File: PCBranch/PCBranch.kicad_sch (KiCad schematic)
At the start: 15 parts, among them J1 CLP-105-02-X-D, J2 DF40HC_3.0_-100DS-0.4V_51_, J3 DF40HC_3.0_-100DS-0.4V_51_, J4 Conn_02x25_Odd_Even, J5 Conn_02x25_Odd_Even, J6 Conn_02x25_Odd_Even, J7 Conn_02x25_Odd_Even

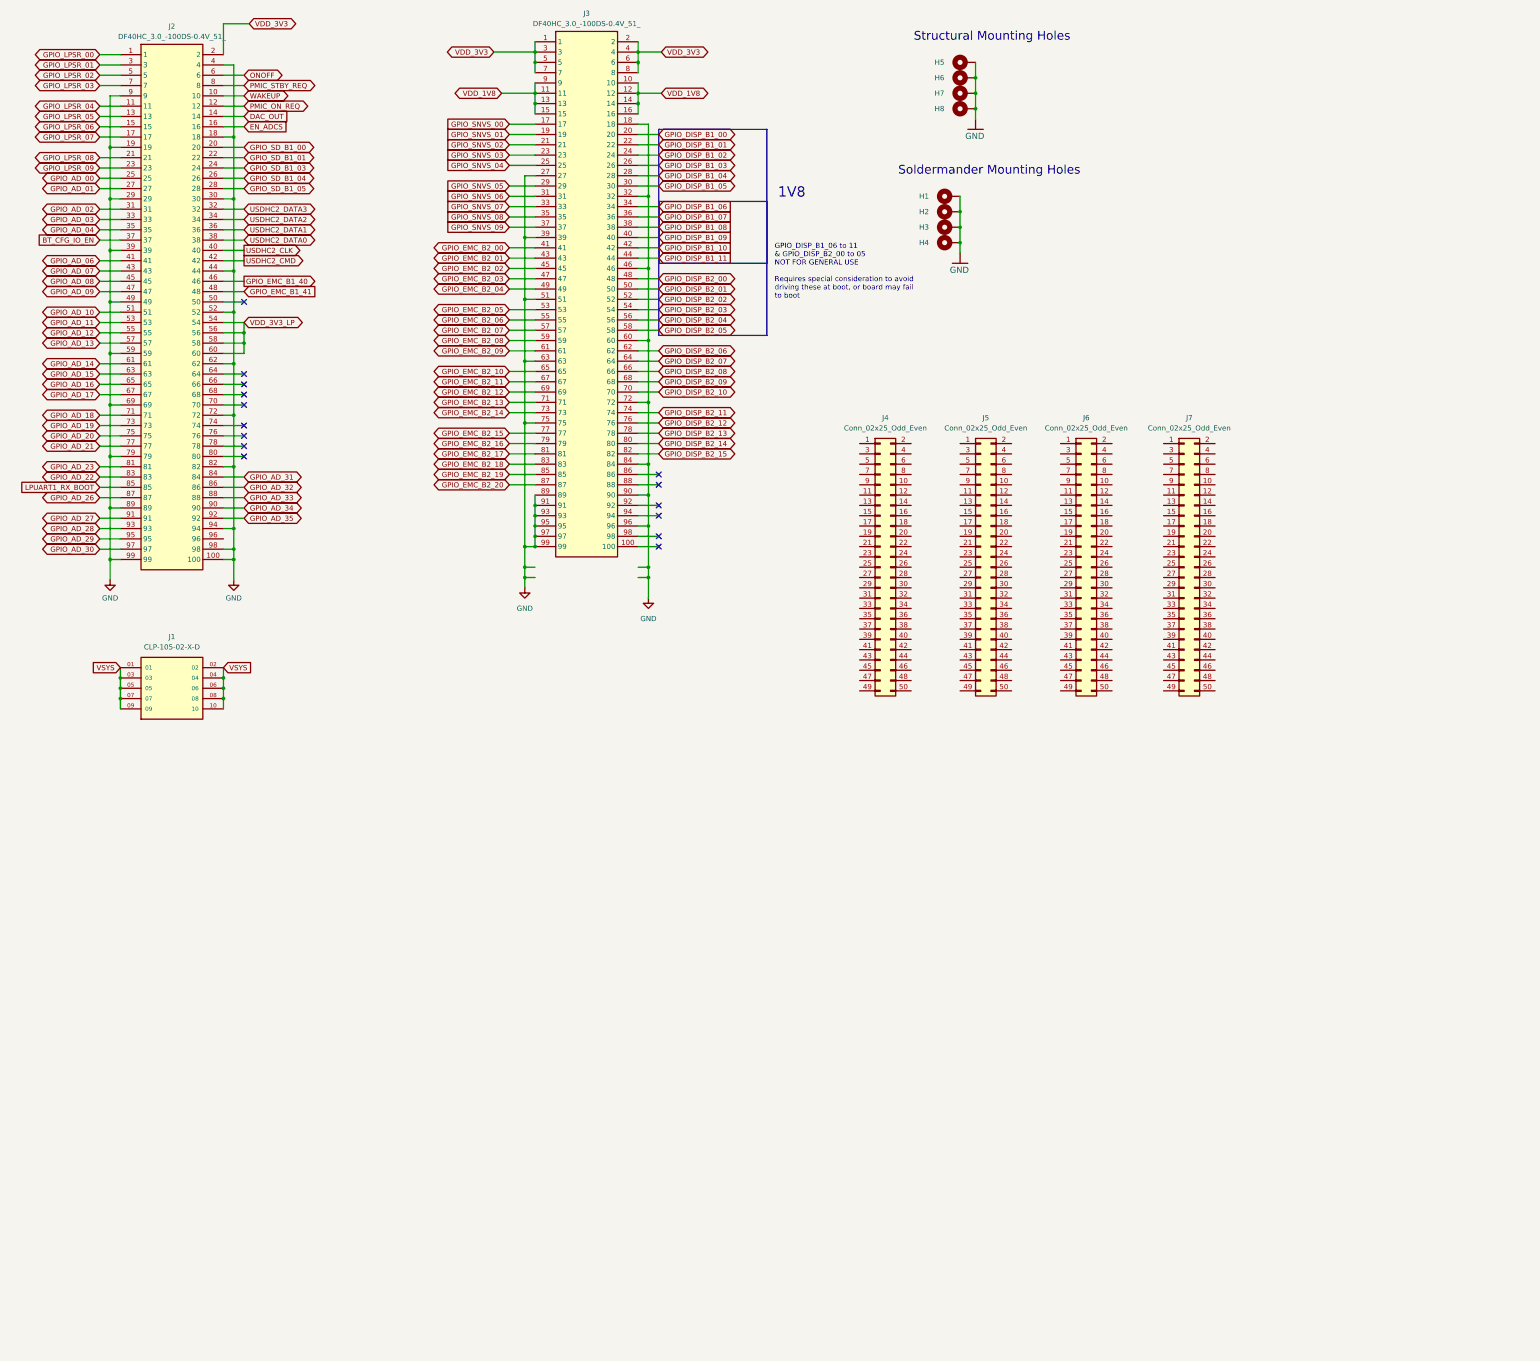
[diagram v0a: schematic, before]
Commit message: PCBranch ready for review
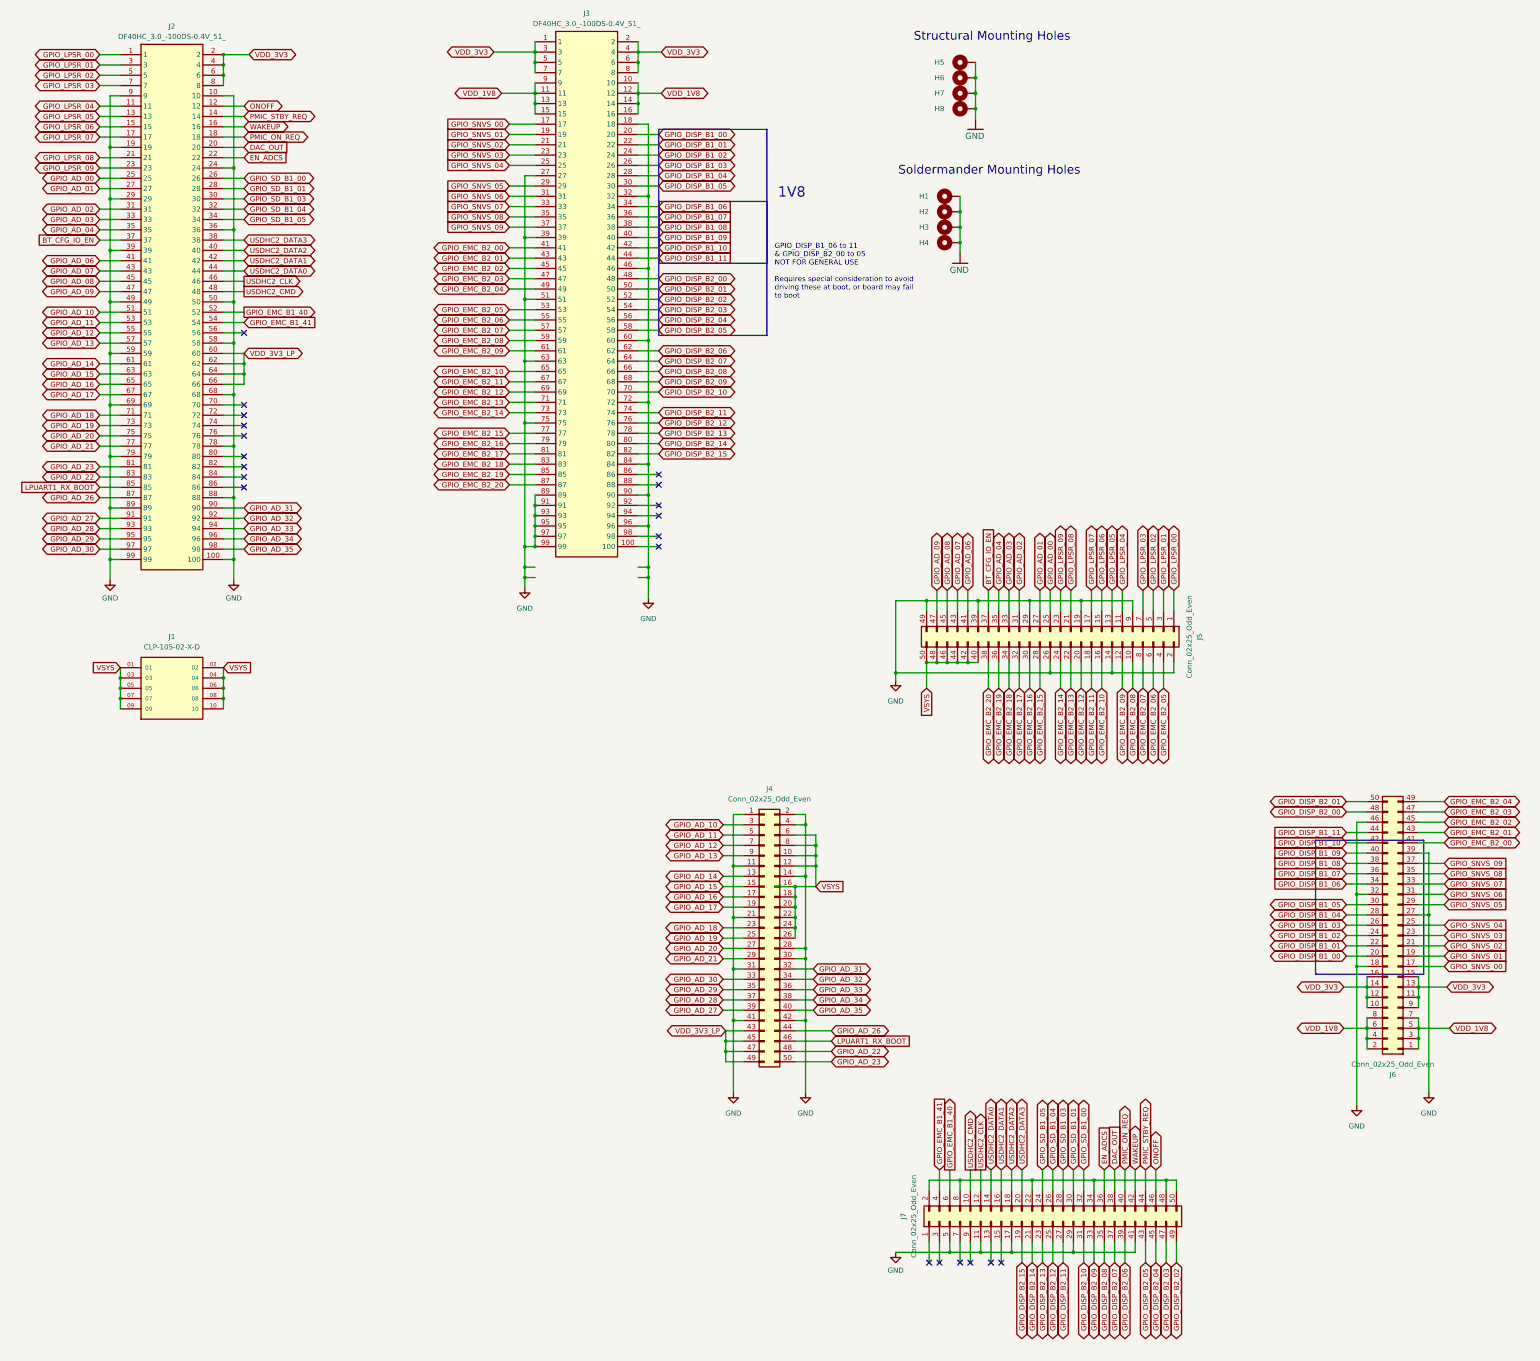
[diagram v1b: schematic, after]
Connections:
- net BT_CFG_IO_EN: now also J5.37 (Pin_37)
- net DAC_OUT: now also J2.20, J7.38 (Pin_38); no longer J2.14
- net EN_ADCS: now also J2.22, J7.36 (Pin_36); no longer J2.16
- net GND: now also J2.10, J2.24, J2.36, J2.50, J2.58, J2.68, J2.78, J2.88, J4.1 (Pin_1), J4.11 (Pin_11), J4.14 (Pin_14), J4.2 (Pin_2), J4.21 (Pin_21), J4.28 (Pin_28), J4.30 (Pin_30), J4.31 (Pin_31), J4.4 (Pin_4), J4.41 (Pin_41), J4.42 (Pin_42), J5.14 (Pin_14), J5.19 (Pin_19), J5.2 (Pin_2), J5.26 (Pin_26), J5.29 (Pin_29), J5.39 (Pin_39), J5.49 (Pin_49), J5.9 (Pin_9), J6.18 (Pin_18), J6.27 (Pin_27), J6.32 (Pin_32), J6.39 (Pin_39), J6.46 (Pin_46), J7.11 (Pin_11), J7.17 (Pin_17), J7.29 (Pin_29), J7.41 (Pin_41), J7.5 (Pin_5); no longer J2.18, J2.30, J2.4, J2.44, J2.52, J2.62, J2.72, J2.82, J2.94, J2.98
- net GPIO_AD_00: now also J5.25 (Pin_25)
- net GPIO_AD_01: now also J5.27 (Pin_27)
- net GPIO_AD_02: now also J5.31 (Pin_31)
- net GPIO_AD_03: now also J5.33 (Pin_33)
- net GPIO_AD_04: now also J5.35 (Pin_35)
- net GPIO_AD_06: now also J5.41 (Pin_41)
- net GPIO_AD_07: now also J5.43 (Pin_43)
- net GPIO_AD_08: now also J5.45 (Pin_45)
- net GPIO_AD_09: now also J5.47 (Pin_47)
- net GPIO_AD_10: now also J4.3 (Pin_3)
- net GPIO_AD_11: now also J4.5 (Pin_5)
- net GPIO_AD_12: now also J4.7 (Pin_7)
- net GPIO_AD_13: now also J4.9 (Pin_9)
- net GPIO_AD_14: now also J4.13 (Pin_13)
- net GPIO_AD_15: now also J4.15 (Pin_15)
- net GPIO_AD_16: now also J4.17 (Pin_17)
- net GPIO_AD_17: now also J4.19 (Pin_19)
- net GPIO_AD_18: now also J4.23 (Pin_23)
- net GPIO_AD_19: now also J4.25 (Pin_25)
- net GPIO_AD_20: now also J4.27 (Pin_27)
- net GPIO_AD_21: now also J4.29 (Pin_29)
- net GPIO_AD_22: now also J4.48 (Pin_48)
- net GPIO_AD_23: now also J4.50 (Pin_50)
- net GPIO_AD_26: now also J4.44 (Pin_44)
- net GPIO_AD_27: now also J4.39 (Pin_39)
- net GPIO_AD_28: now also J4.37 (Pin_37)
- net GPIO_AD_29: now also J4.35 (Pin_35)
- net GPIO_AD_30: now also J4.33 (Pin_33)
- net GPIO_AD_31: now also J2.90, J4.32 (Pin_32); no longer J2.84
- net GPIO_AD_32: now also J2.92, J4.34 (Pin_34); no longer J2.86
- net GPIO_AD_33: now also J2.94, J4.36 (Pin_36); no longer J2.88
- net GPIO_AD_34: now also J2.96, J4.38 (Pin_38); no longer J2.90
- net GPIO_AD_35: now also J2.98, J4.40 (Pin_40); no longer J2.92
- net GPIO_DISP_B1_00: now also J6.20 (Pin_20)
- net GPIO_DISP_B1_01: now also J6.22 (Pin_22)
- net GPIO_DISP_B1_02: now also J6.24 (Pin_24)
- net GPIO_DISP_B1_03: now also J6.26 (Pin_26)
- net GPIO_DISP_B1_04: now also J6.28 (Pin_28)
- net GPIO_DISP_B1_05: now also J6.30 (Pin_30)
- net GPIO_DISP_B1_06: now also J6.34 (Pin_34)
- net GPIO_DISP_B1_07: now also J6.36 (Pin_36)
- net GPIO_DISP_B1_08: now also J6.38 (Pin_38)
- net GPIO_DISP_B1_09: now also J6.40 (Pin_40)
- net GPIO_DISP_B1_10: now also J6.42 (Pin_42)
- net GPIO_DISP_B1_11: now also J6.44 (Pin_44)
- net GPIO_DISP_B2_00: now also J6.48 (Pin_48)
- net GPIO_DISP_B2_01: now also J6.50 (Pin_50)
- net GPIO_DISP_B2_02: now also J7.49 (Pin_49)
- net GPIO_DISP_B2_03: now also J7.47 (Pin_47)
- net GPIO_DISP_B2_04: now also J7.45 (Pin_45)
- net GPIO_DISP_B2_05: now also J7.43 (Pin_43)
- net GPIO_DISP_B2_06: now also J7.39 (Pin_39)
- net GPIO_DISP_B2_07: now also J7.37 (Pin_37)
- net GPIO_DISP_B2_08: now also J7.35 (Pin_35)
- net GPIO_DISP_B2_09: now also J7.33 (Pin_33)
- net GPIO_DISP_B2_10: now also J7.31 (Pin_31)
- net GPIO_DISP_B2_11: now also J7.27 (Pin_27)
- net GPIO_DISP_B2_12: now also J7.25 (Pin_25)
- net GPIO_DISP_B2_13: now also J7.23 (Pin_23)
- net GPIO_DISP_B2_14: now also J7.21 (Pin_21)
- net GPIO_DISP_B2_15: now also J7.19 (Pin_19)
- net GPIO_EMC_B1_40: now also J2.52, J7.6 (Pin_6); no longer J2.46
- net GPIO_EMC_B1_41: now also J2.54, J7.4 (Pin_4); no longer J2.48
- net GPIO_EMC_B2_00: now also J6.41 (Pin_41)
- net GPIO_EMC_B2_01: now also J6.43 (Pin_43)
- net GPIO_EMC_B2_02: now also J6.45 (Pin_45)
- net GPIO_EMC_B2_03: now also J6.47 (Pin_47)
- net GPIO_EMC_B2_04: now also J6.49 (Pin_49)
- net GPIO_EMC_B2_05: now also J5.4 (Pin_4)
- net GPIO_EMC_B2_06: now also J5.6 (Pin_6)
- net GPIO_EMC_B2_07: now also J5.8 (Pin_8)
- net GPIO_EMC_B2_08: now also J5.10 (Pin_10)
- net GPIO_EMC_B2_09: now also J5.12 (Pin_12)
- net GPIO_EMC_B2_10: now also J5.16 (Pin_16)
- net GPIO_EMC_B2_11: now also J5.18 (Pin_18)
- net GPIO_EMC_B2_12: now also J5.20 (Pin_20)
- net GPIO_EMC_B2_13: now also J5.22 (Pin_22)
- net GPIO_EMC_B2_14: now also J5.24 (Pin_24)
- net GPIO_EMC_B2_15: now also J5.28 (Pin_28)
- net GPIO_EMC_B2_16: now also J5.30 (Pin_30)
- net GPIO_EMC_B2_17: now also J5.32 (Pin_32)
- net GPIO_EMC_B2_18: now also J5.34 (Pin_34)
- net GPIO_EMC_B2_19: now also J5.36 (Pin_36)
- net GPIO_EMC_B2_20: now also J5.38 (Pin_38)
- net GPIO_LPSR_00: now also J5.1 (Pin_1)
- net GPIO_LPSR_01: now also J5.3 (Pin_3)
- net GPIO_LPSR_02: now also J5.5 (Pin_5)
- net GPIO_LPSR_03: now also J5.7 (Pin_7)
- net GPIO_LPSR_04: now also J5.11 (Pin_11)
- net GPIO_LPSR_05: now also J5.13 (Pin_13)
- net GPIO_LPSR_06: now also J5.15 (Pin_15)
- net GPIO_LPSR_07: now also J5.17 (Pin_17)
- net GPIO_LPSR_08: now also J5.21 (Pin_21)
- net GPIO_LPSR_09: now also J5.23 (Pin_23)
- net GPIO_SD_B1_00: now also J2.26, J7.32 (Pin_32); no longer J2.20
- net GPIO_SD_B1_01: now also J2.28, J7.30 (Pin_30); no longer J2.22
- net GPIO_SD_B1_03: now also J2.30, J7.28 (Pin_28); no longer J2.24
- net GPIO_SD_B1_04: now also J2.32, J7.26 (Pin_26); no longer J2.26
- net GPIO_SD_B1_05: now also J2.34, J7.24 (Pin_24); no longer J2.28
- net GPIO_SNVS_00: now also J6.17 (Pin_17)
- net GPIO_SNVS_01: now also J6.19 (Pin_19)
- net GPIO_SNVS_02: now also J6.21 (Pin_21)
- net GPIO_SNVS_03: now also J6.23 (Pin_23)
- net GPIO_SNVS_04: now also J6.25 (Pin_25)
- net GPIO_SNVS_05: now also J6.29 (Pin_29)
- net GPIO_SNVS_06: now also J6.31 (Pin_31)
- net GPIO_SNVS_07: now also J6.33 (Pin_33)
- net GPIO_SNVS_08: now also J6.35 (Pin_35)
- net GPIO_SNVS_09: now also J6.37 (Pin_37)
- net LPUART1_RX_BOOT: now also J4.46 (Pin_46)
- net ONOFF: now also J2.12, J7.46 (Pin_46); no longer J2.6
- net PMIC_ON_REQ: now also J2.18, J7.40 (Pin_40); no longer J2.12
- net PMIC_STBY_REQ: now also J2.14, J7.44 (Pin_44); no longer J2.8
- net USDHC2_CLK: now also J2.46, J7.12 (Pin_12); no longer J2.40
- net USDHC2_CMD: now also J2.48, J7.10 (Pin_10); no longer J2.42
- net USDHC2_DATA0: now also J2.44, J7.14 (Pin_14); no longer J2.38
- net USDHC2_DATA1: now also J2.42, J7.16 (Pin_16); no longer J2.36
- net USDHC2_DATA2: now also J2.40, J7.18 (Pin_18); no longer J2.34
- net USDHC2_DATA3: now also J2.38, J7.20 (Pin_20); no longer J2.32
- net VDD_1V8: now also J6.1 (Pin_1), J6.2 (Pin_2), J6.3 (Pin_3), J6.4 (Pin_4), J6.5 (Pin_5), J6.6 (Pin_6), J6.7 (Pin_7), J6.8 (Pin_8)
- net VDD_3V3: now also J2.4, J2.6, J2.8, J6.10 (Pin_10), J6.11 (Pin_11), J6.12 (Pin_12), J6.13 (Pin_13), J6.14 (Pin_14), J6.15 (Pin_15), J6.16 (Pin_16), J6.9 (Pin_9)
- net VDD_3V3_LP: now also J2.62, J2.64, J2.66, J4.43 (Pin_43), J4.45 (Pin_45), J4.47 (Pin_47), J4.49 (Pin_49); no longer J2.54, J2.56, J2.58
- net VSYS: now also J4.10 (Pin_10), J4.12 (Pin_12), J4.16 (Pin_16), J4.18 (Pin_18), J4.20 (Pin_20), J4.22 (Pin_22), J4.24 (Pin_24), J4.26 (Pin_26), J4.6 (Pin_6), J4.8 (Pin_8), J5.40 (Pin_40), J5.42 (Pin_42), J5.44 (Pin_44), J5.46 (Pin_46), J5.48 (Pin_48), J5.50 (Pin_50)
- net WAKEUP: now also J2.16, J7.42 (Pin_42); no longer J2.10
- net at J7.2 (Pin_2): now also J7.22 (Pin_22), J7.34 (Pin_34), J7.48 (Pin_48), J7.50 (Pin_50), J7.8 (Pin_8)
- no-connect marks 15 -> 21
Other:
- moved on the sheet: J4, J5, J6, J7
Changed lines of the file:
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@@
 (kicad_sch (version 20230121) (generator eeschema)
-  (paper "A3")
+  (paper "A2")
